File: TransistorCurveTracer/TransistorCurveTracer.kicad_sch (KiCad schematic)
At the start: 24 parts, among them J1 Conn_01x04_Pin, J2 Conn_01x04_Pin, J3 Conn_01x04_Pin, Q1 BC547, U1 NE555P, U3 MCP601-xP

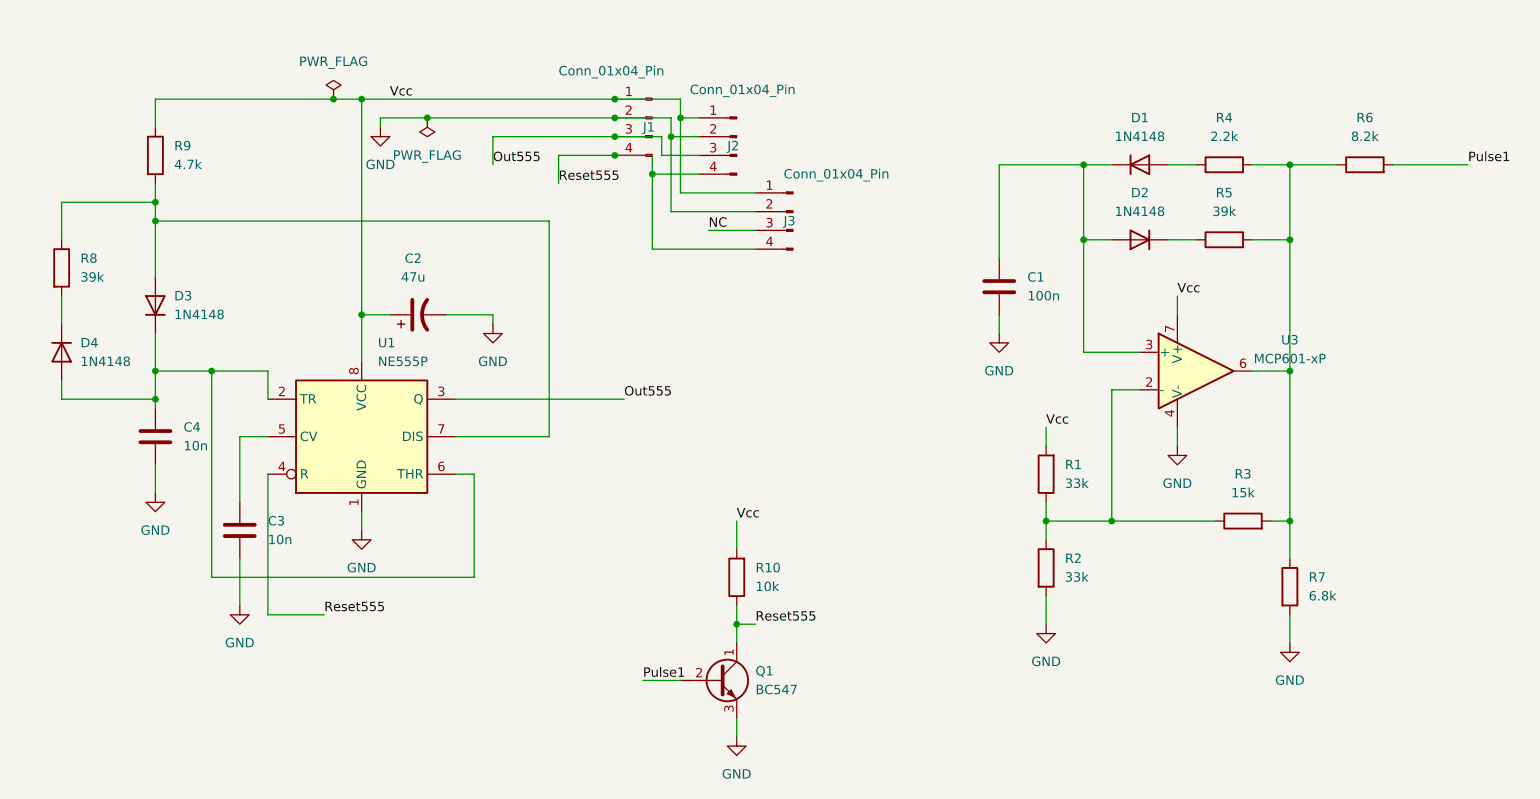
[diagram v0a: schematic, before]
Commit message: in progress
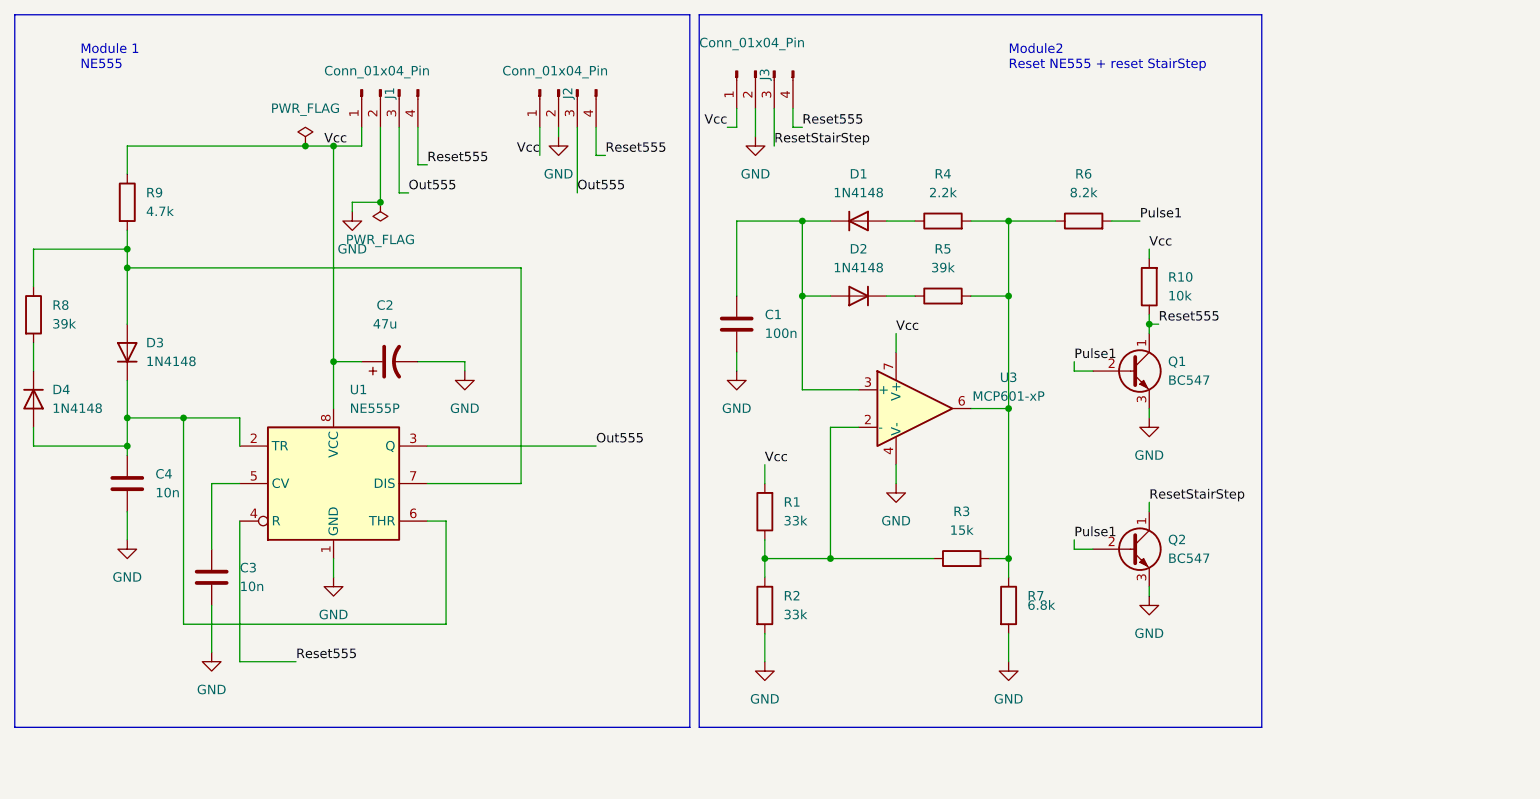
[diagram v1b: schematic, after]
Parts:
- added Q2: BC547, Package_TO_SOT_THT:TO-92_Inline, symbol Transistor_BJT:BC547
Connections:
- net GND: now also Q2.3 (E)
- net Pulse1: now also Q2.2 (B)
- net NC renamed ResetStairStep
- net ResetStairStep: now also Q2.1 (C)
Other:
- note added: "Module 1 NE555"
- note added: "Module2 Reset NE555 + reset StairStep"
- moved on the sheet: C1, C2, C3, C4, D1, D2, D3, D4, J1, J2, J3, Q1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
